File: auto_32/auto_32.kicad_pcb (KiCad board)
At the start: 4 copper layers, 82.6 x 101.6 mm, 11 parts, among them J3 USB_C_Receptacle_USB2.0_16P, SW1 SW_Push, U2 CH343P, U2 ESP32-S3-WROOM-1, U5 CH334F

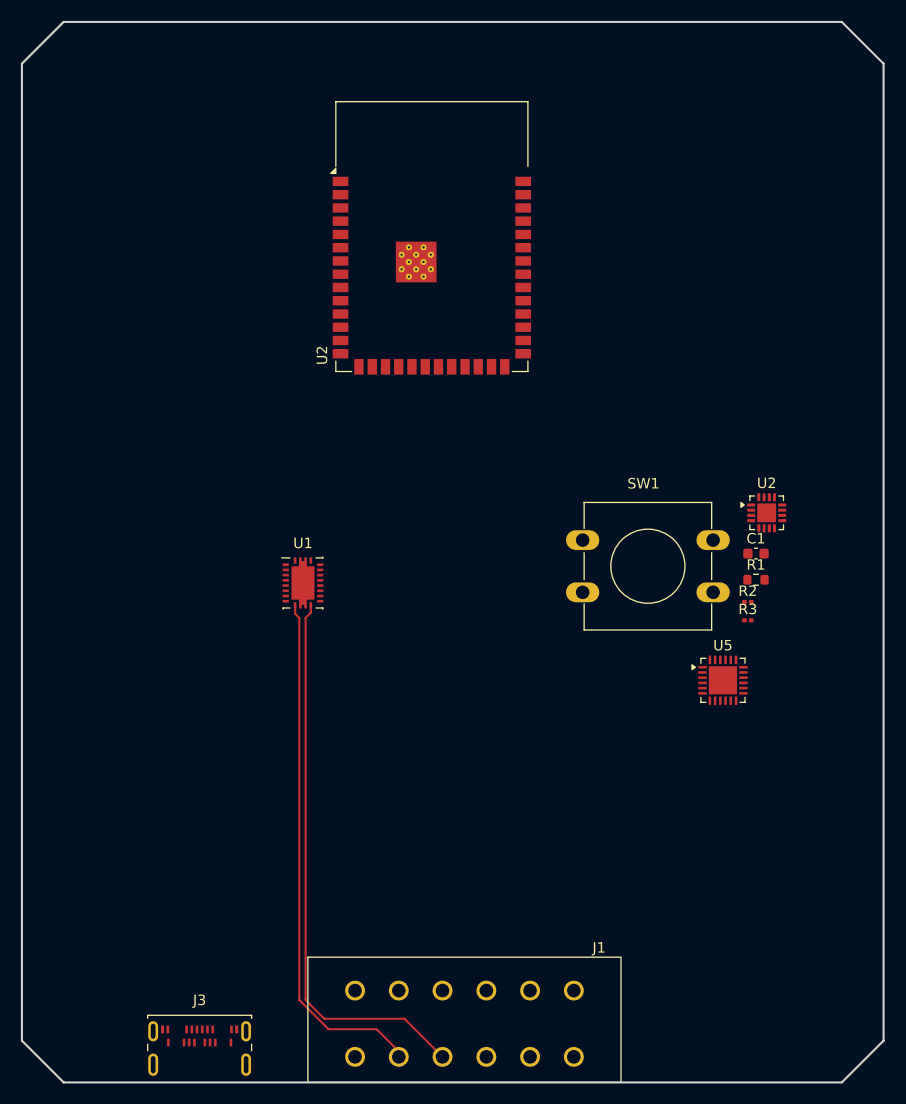
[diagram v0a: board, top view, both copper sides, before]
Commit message: march update
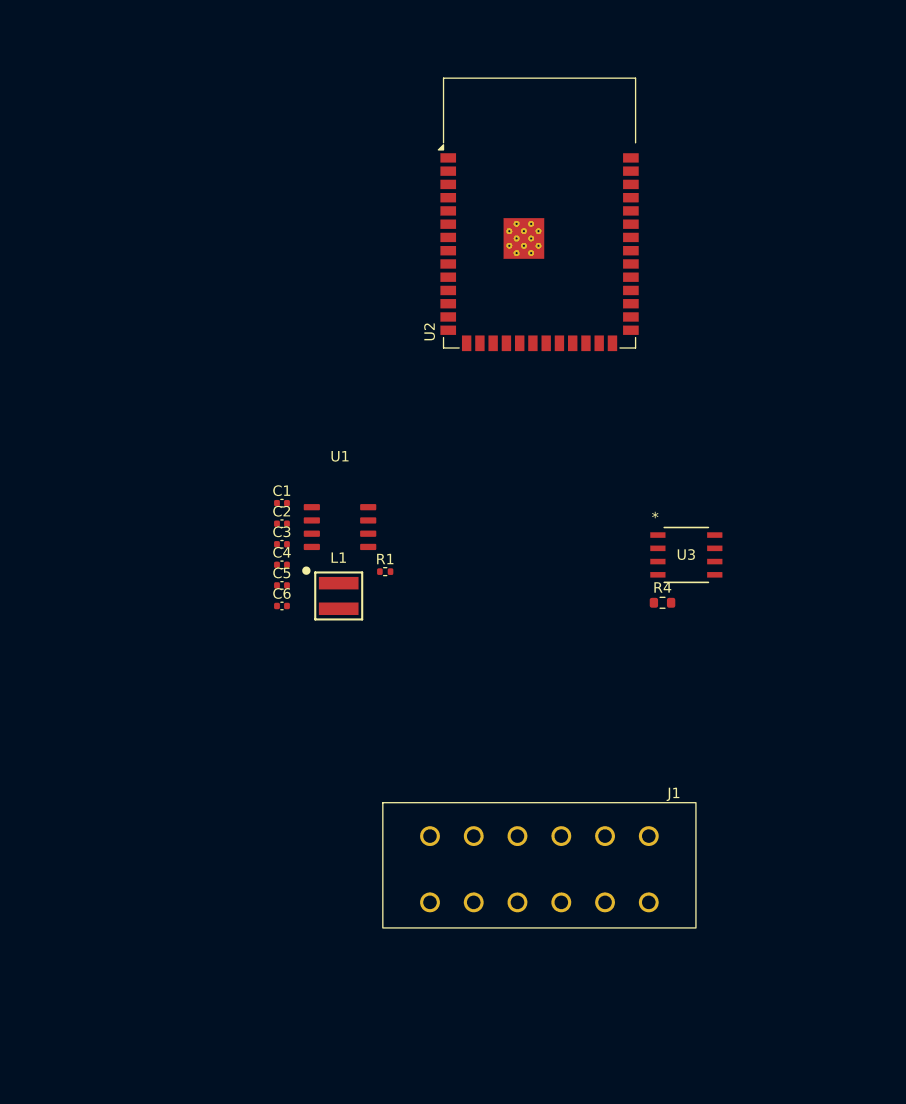
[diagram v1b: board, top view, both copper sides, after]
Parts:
- removed J3: USB_C_Receptacle_USB2.0_16P, Connector_USB:USB_C_Receptacle_Amphenol_124019772112A
- removed R2, R3: 5.1k, Resistor_SMD:R_0201_0603Metric
- removed SW1: SW_Push, Button_Switch_THT:SW_PUSH-12mm
- removed the U2 at (119.6, 98.5)
- removed the U2 at (87.5, 72.0)
- removed U5: CH334F, Package_DFN_QFN:QFN-24-1EP_4x4mm_P0.5mm_EP2.7x2.7mm
- added C2: C, Capacitor_SMD:C_0402_1005Metric, F.Cu at (73.1, 99.6)
- added C3: C, Capacitor_SMD:C_0402_1005Metric, F.Cu at (73.1, 101.5)
- added C4: C, Capacitor_SMD:C_0402_1005Metric, F.Cu at (73.1, 103.5)
- added C5: C, Capacitor_SMD:C_0402_1005Metric, F.Cu at (73.1, 105.5)
- added C6: C, Capacitor_SMD:C_0402_1005Metric, F.Cu at (73.1, 107.5)
- added L1: WE-XHMI_4040, ssh_DISC_lib:WE-XHMI_4040, F.Cu at (78.6, 106.5)
- added R4: 0, Resistor_SMD:R_0603_1608Metric, F.Cu at (109.6, 107.1)
- added U2: ESP32-S3-WROOM-1, RF_Module:ESP32-S3-WROOM-1, F.Cu at (97.8, 69.8)
- added U3: TJA1051T/3/1J, ssh_IC_FP:SO8_SOT96-1_NXP, F.Cu at (111.9, 102.6)
- C1: footprint Capacitor_SMD:C_0603_1608Metric -> Capacitor_SMD:C_0402_1005Metric
- R1: footprint Resistor_SMD:R_0603_1608Metric -> Resistor_SMD:R_0402_1005Metric
- U1: footprint ssh_Library:VQFN-26_EP_3.5x4.5_Pitch0.5mm -> ssh_IC_FP:SOIC_8
- moved C1 45.7 mm to (73.1, 97.6)
- moved R1 35.5 mm to (83.0, 104.2)
- moved J1 16.4 mm to (97.8, 138.3)
- moved U1 6.42 mm to (78.7, 99.9)
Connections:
- C1 pad 1: Net-(C1-Pad1) -> Net-(U1-Vin)
- C1 pad 2: GND -> Net-(U1-GND)
- J1 pad 1: Net-(U4-IO3) -> unconnected-(J1-Pad1)
- J1 pad 2: Net-(U4-IO46) -> unconnected-(J1-Pad2)
- J1 pad 4: Net-(U1-CANH) -> unconnected-(J1-Pad4)
- J1 pad 5: Net-(U1-CANL) -> unconnected-(J1-Pad5)
- R1 pad 1: Net-(C1-Pad1) -> Net-(U1-COMP)
- R1 pad 2: /EN -> Net-(C3-Pad1)
- U1 pad 1: unconnected-(U1-OSC1-Pad1) -> Net-(U1-BOOT)
- U1 pad 2: unconnected-(U1-nWKRQ-Pad2) -> (no net)
- U1 pad 4: unconnected-(U1-SCLK-Pad4) -> Net-(U1-SS)
- U1 pad 6: unconnected-(U1-SDO-Pad6) -> Net-(U1-COMP)
- U1 pad 7: unconnected-(U1-nCS-Pad7) -> Net-(U1-GND)
- U1 pad 8: unconnected-(U1-nINT-Pad8) -> Net-(U1-PH)
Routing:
- net Net-(U1-CANH): track 53.4 -> 0.00 mm
- net Net-(U1-CANL): track 50.1 -> 0.00 mm
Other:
- board outline removed
